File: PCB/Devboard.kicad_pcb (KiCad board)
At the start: 2 copper layers, 556 parts, among them Q1 IPB180P04P4L-02, Q2 IPB180P04P4L-02, SW1 SW_Push, U1 TVS2201DRBR, U10 TPS62822DLCR, U11 TPS62823DLCR, U12 TPS548A20RVER, U13 TPS7A4700RGWR, U14 TPS3700DSET, U15 TPS54824RNVR, U16 TPS54824RNVR, U17 TPS7A4700RGWR, U18 DW06, U19 TPS61088RHLR, U2 TPD6S300ARUKR, U20 TPS54824RNVR, U21 LM66100DCK, U22 TPS7A4700RGWR, U23 TPS7A4700RGWR, U24 TPS259470ARPWR, U25 TPS54824RNVR, U26 xczu4evfbvb900pkg, U27 RS3112-1.25XSF3, U3 STUSB4500QTR, U32 USB3320C-EZK-TR, U33 USBLC6-2SC6, U34 CP2102N-Axx-xQFN24, U35 TXB0108PW, U36 TCA9548APWR, U37 PCA9306, U4 TPS2121RUXR, U5 TPS259470ARPWR, U6 BQ25895RTWR, U7 BQ27441DRZR-G1A, U8 TPS62130RGTR, U9 XT60, Y1 25 MHz, Y2 25 MHz

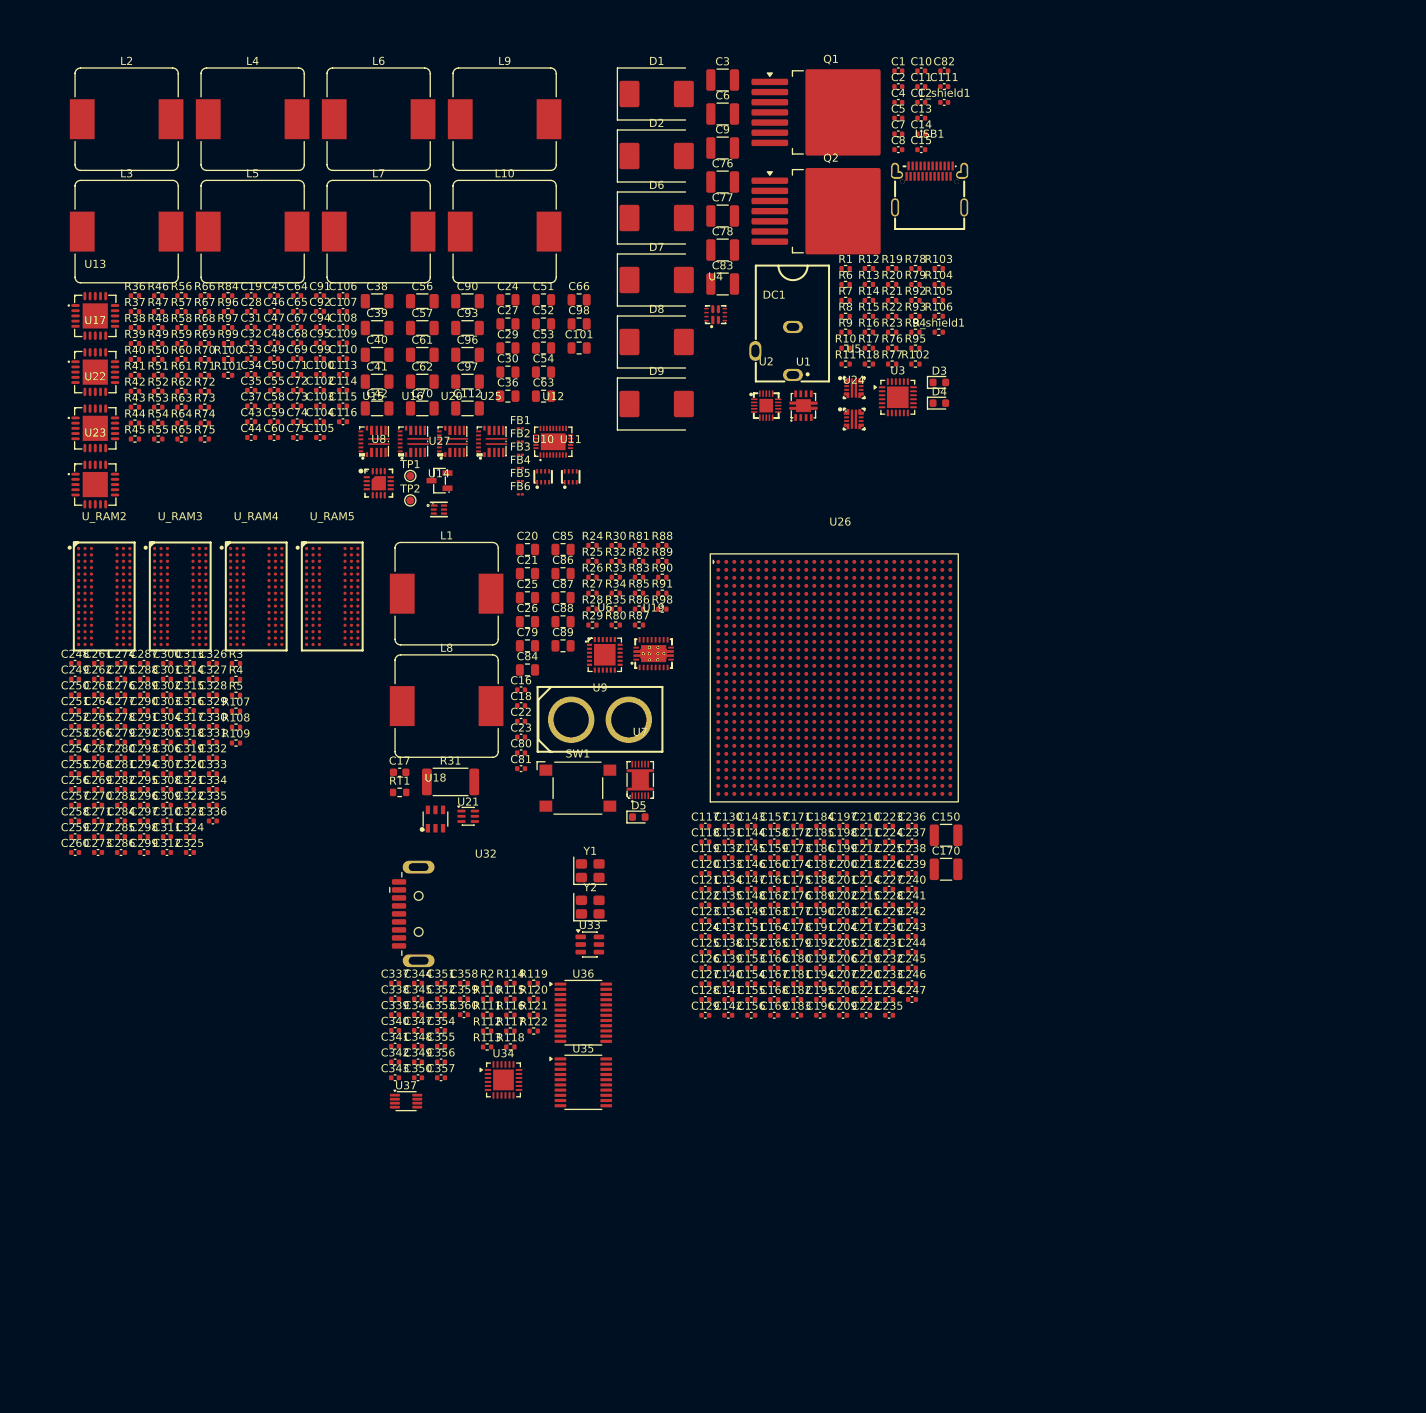
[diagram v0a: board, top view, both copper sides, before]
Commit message: Feat : Completed 04d Peripherals
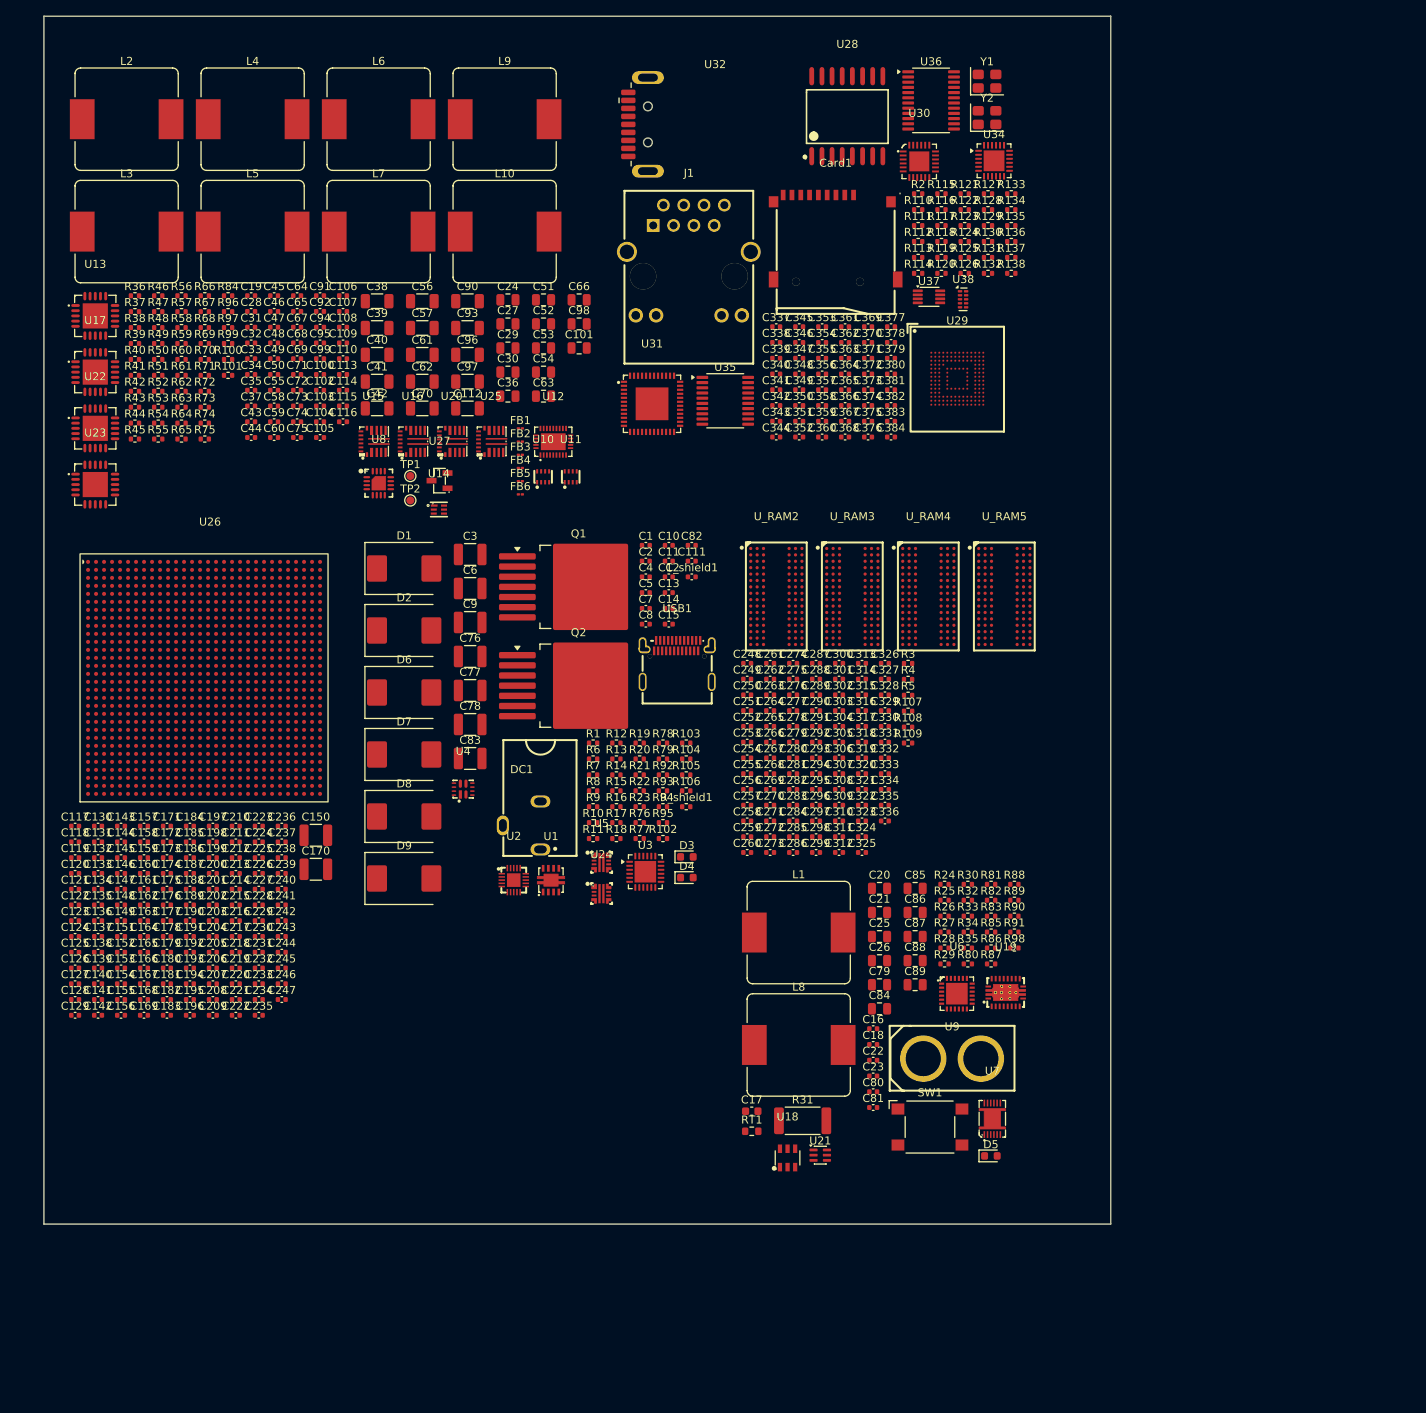
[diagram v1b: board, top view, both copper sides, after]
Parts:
- removed U33: USBLC6-2SC6, Package_TO_SOT_SMD:SOT-23-6
- added C361: 0.1uF, Capacitor_SMD:C_0402_1005Metric, F.Cu at (97.2, 32.5)
- added C362: 0.1uF, Capacitor_SMD:C_0402_1005Metric, F.Cu at (97.2, 34.4)
- added C363: 0.1uF, Capacitor_SMD:C_0402_1005Metric, F.Cu at (97.2, 36.4)
- added C364: 1nF, Capacitor_SMD:C_0402_1005Metric, F.Cu at (97.2, 38.4)
- added C365: 1nF, Capacitor_SMD:C_0402_1005Metric, F.Cu at (97.2, 40.3)
- added C366: 1nF, Capacitor_SMD:C_0402_1005Metric, F.Cu at (97.2, 42.3)
- added C367: 0.1uF, Capacitor_SMD:C_0402_1005Metric, F.Cu at (97.2, 44.3)
- added C368: 1nF, Capacitor_SMD:C_0402_1005Metric, F.Cu at (97.2, 46.3)
- added C369: 0.1uF, Capacitor_SMD:C_0402_1005Metric, F.Cu at (100.1, 32.5)
- added C370: 1nF, Capacitor_SMD:C_0402_1005Metric, F.Cu at (100.1, 34.4)
- added C371: 0.1uF, Capacitor_SMD:C_0402_1005Metric, F.Cu at (100.1, 36.4)
- added C372: 1nF, Capacitor_SMD:C_0402_1005Metric, F.Cu at (100.1, 38.4)
- added C373: 0.1uF, Capacitor_SMD:C_0402_1005Metric, F.Cu at (100.1, 40.3)
- added C374: 1nF, Capacitor_SMD:C_0402_1005Metric, F.Cu at (100.1, 42.3)
- added C375: 22uF, Capacitor_SMD:C_0402_1005Metric, F.Cu at (100.1, 44.3)
- added C376: 22uF, Capacitor_SMD:C_0402_1005Metric, F.Cu at (100.1, 46.3)
- added C377: 0.1uF, Capacitor_SMD:C_0402_1005Metric, F.Cu at (102.9, 32.5)
- added C378: 0.1uF, Capacitor_SMD:C_0402_1005Metric, F.Cu at (102.9, 34.4)
- added C379: 22uF, Capacitor_SMD:C_0402_1005Metric, F.Cu at (102.9, 36.4)
- added C380: 22uF, Capacitor_SMD:C_0402_1005Metric, F.Cu at (102.9, 38.4)
- added C381: 0.1uF, Capacitor_SMD:C_0402_1005Metric, F.Cu at (102.9, 40.3)
- added C382: 0.1uF, Capacitor_SMD:C_0402_1005Metric, F.Cu at (102.9, 42.3)
- added C383: 0.1uF, Capacitor_SMD:C_0402_1005Metric, F.Cu at (102.9, 44.3)
- added C384: 0.1uF, Capacitor_SMD:C_0402_1005Metric, F.Cu at (102.9, 46.3)
- added Card1: TF-01A, Devboard_Footprints:TF-SMD_TF-01A, F.Cu at (96.0, 21.3)
- added J1: HR911105A_C12074, Devboard_Footprints:RJ45-TH_HR911105A, F.Cu at (77.7, 24.2)
- added R123: 22Ω, Resistor_SMD:R_0402_1005Metric, F.Cu at (112.1, 19.8)
- added R124: 22Ω, Resistor_SMD:R_0402_1005Metric, F.Cu at (112.1, 21.8)
- added R125: 22Ω, Resistor_SMD:R_0402_1005Metric, F.Cu at (112.1, 23.8)
- added R126: 22Ω, Resistor_SMD:R_0402_1005Metric, F.Cu at (112.1, 25.8)
- added R127: 22Ω, Resistor_SMD:R_0402_1005Metric, F.Cu at (115.0, 15.8)
- added R128: 22Ω, Resistor_SMD:R_0402_1005Metric, F.Cu at (115.0, 17.8)
- added R129: 22Ω, Resistor_SMD:R_0402_1005Metric, F.Cu at (115.0, 19.8)
- added R130: 22Ω, Resistor_SMD:R_0402_1005Metric, F.Cu at (115.0, 21.8)
- added R131: 10kΩ, Resistor_SMD:R_0402_1005Metric, F.Cu at (115.0, 23.8)
- added R132: 10kΩ, Resistor_SMD:R_0402_1005Metric, F.Cu at (115.0, 25.8)
- added R133: 2.49kΩ, Resistor_SMD:R_0402_1005Metric, F.Cu at (118.0, 15.8)
- added R134: 10kΩ, Resistor_SMD:R_0402_1005Metric, F.Cu at (118.0, 17.8)
- added R135: 2.49kΩ, Resistor_SMD:R_0402_1005Metric, F.Cu at (118.0, 19.8)
- added R136: 11kΩ, Resistor_SMD:R_0402_1005Metric, F.Cu at (118.0, 21.8)
- added R137: 470Ω, Resistor_SMD:R_0402_1005Metric, F.Cu at (118.0, 23.8)
- added R138: 470Ω, Resistor_SMD:R_0402_1005Metric, F.Cu at (118.0, 25.8)
- added U28: MT25QU256ABA8ESF-0SIT TR, Devboard_Footprints:SOP-16_L10.3-W7.5-P1.27-LS10.4-BL, F.Cu at (97.5, 6.15)
- added U29: FEMDNN032G-A3A55, Devboard_Footprints:FBGA-153_L13.0-W11.5-P0.50_KLMAG1JETD-B041, F.Cu at (111.2, 39.0)
- added U30: TXS02612RTWR, Devboard_Footprints:WQFN-24_L4.0-W4.0-P0.50-TL-EP2.5, F.Cu at (106.5, 11.8)
- added U31: DP83867IRRGZR, Devboard_Footprints:VQFN-48_L7.0-W7.0-P0.50-TL-EP4.1, F.Cu at (73.0, 42.1)
- added U38: TPD4E05U06DQA, Package_SON:USON-10_2.5x1.0mm_P0.5mm, F.Cu at (111.9, 29.0)
- moved U34 130.2 mm to (115.8, 11.7)
- moved U36 122.0 mm to (107.9, 4.17)
- moved U37 119.9 mm to (107.7, 28.7)
- moved R121 115.9 mm to (112.1, 15.8)
- moved R122 115.9 mm to (112.1, 17.8)
- moved R115 114.2 mm to (109.2, 15.8)
- moved R116 114.2 mm to (109.2, 17.8)
- moved R118 114.2 mm to (109.2, 21.8)
- moved R117 114.2 mm to (109.2, 19.8)
- moved R110 112.4 mm to (106.3, 17.8)
- moved R111 112.4 mm to (106.3, 19.8)
- moved R112 112.4 mm to (106.3, 21.8)
- moved R113 112.4 mm to (106.3, 23.8)
- moved R2 112.4 mm to (106.3, 15.8)
- moved Y1 110.5 mm to (114.9, 1.77)
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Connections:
- U26 pad C23: unconnected-(U26-PS_MIO38-PadC23) -> GEM_RST
- U34 pad 2: Net-(U34-GND-Pad2) -> GND
- U34 pad 25: Net-(U34-GND-Pad2) -> GND
- U34 pad 8: unconnected-(U34-VBUS-Pad8) -> VBUS
- U35 pad 11: unconnected-(U35-GND-Pad11) -> GND
- U37 pad 1: unconnected-(U37-GND-Pad1) -> GND
- Y1 pad 1: unconnected-(Y1-Pad1) -> Net-(U31-X_I)
- Y1 pad 2: Net-(Y1-G-Pad2) -> GND
- Y1 pad 3: unconnected-(Y1-Pad3) -> Net-(U31-X_O)
- Y1 pad 4: Net-(Y1-G-Pad2) -> GND
- Y2 pad 1: unconnected-(Y2-Pad1) -> Net-(C380-Pad2)
- Y2 pad 2: Net-(Y2-G-Pad2) -> GND
- Y2 pad 3: unconnected-(Y2-Pad3) -> Net-(C379-Pad2)
- Y2 pad 4: Net-(Y2-G-Pad2) -> GND
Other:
- board outline added: 133.4 x 151 mm
